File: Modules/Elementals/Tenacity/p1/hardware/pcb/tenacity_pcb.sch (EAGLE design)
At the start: 25 parts, among them J1 EURO_POWER, J2 WQP-PJ398SM6, J3 WQP-PJ398SM6, J4 WQP-PJ398SM6, J5 WQP-PJ398SM6, J6 WQP-PJ398SM6, J7 WQP-PJ398SM6, J8 WQP-PJ398SM6, J9 WQP-PJ398SM6, U1 TL072P, U2 TL072P

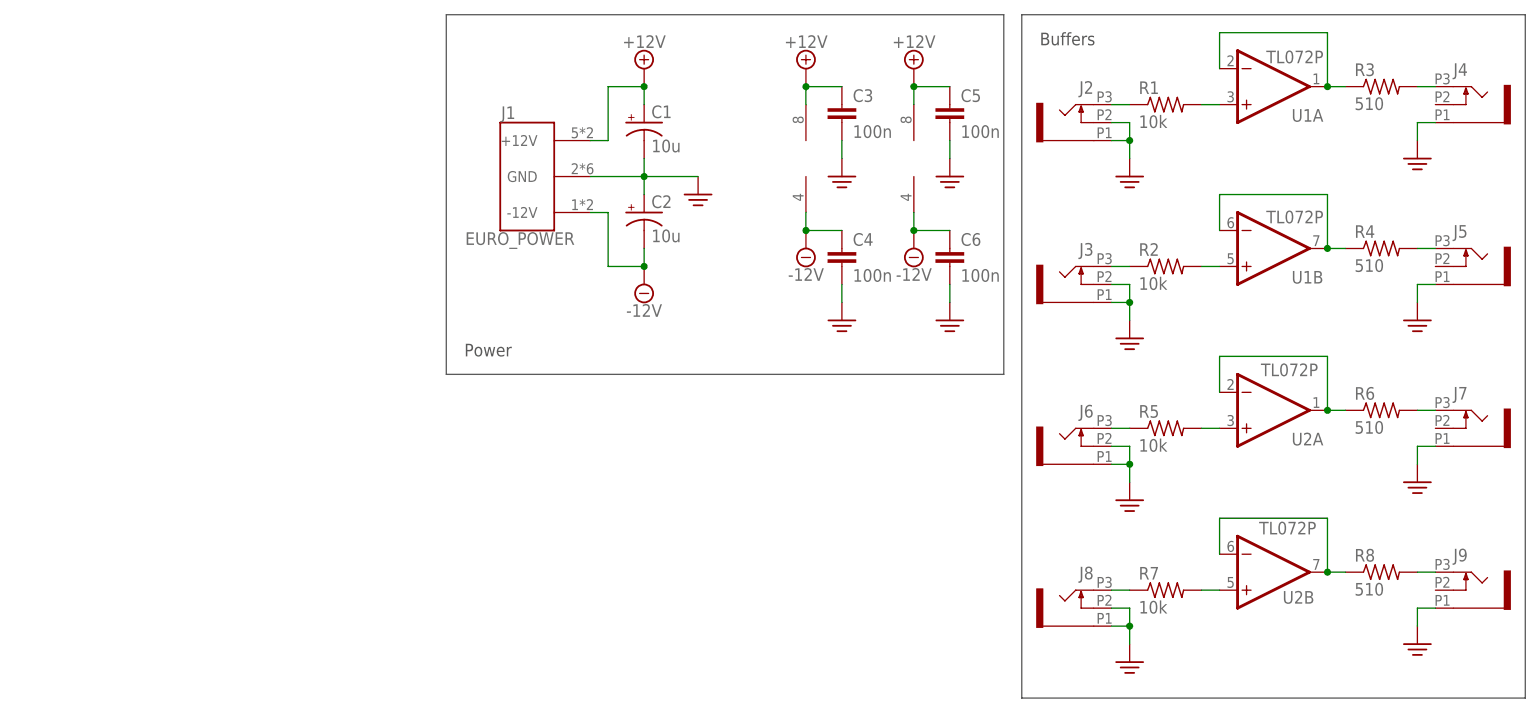
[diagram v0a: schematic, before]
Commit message: Finalized tenacity p1
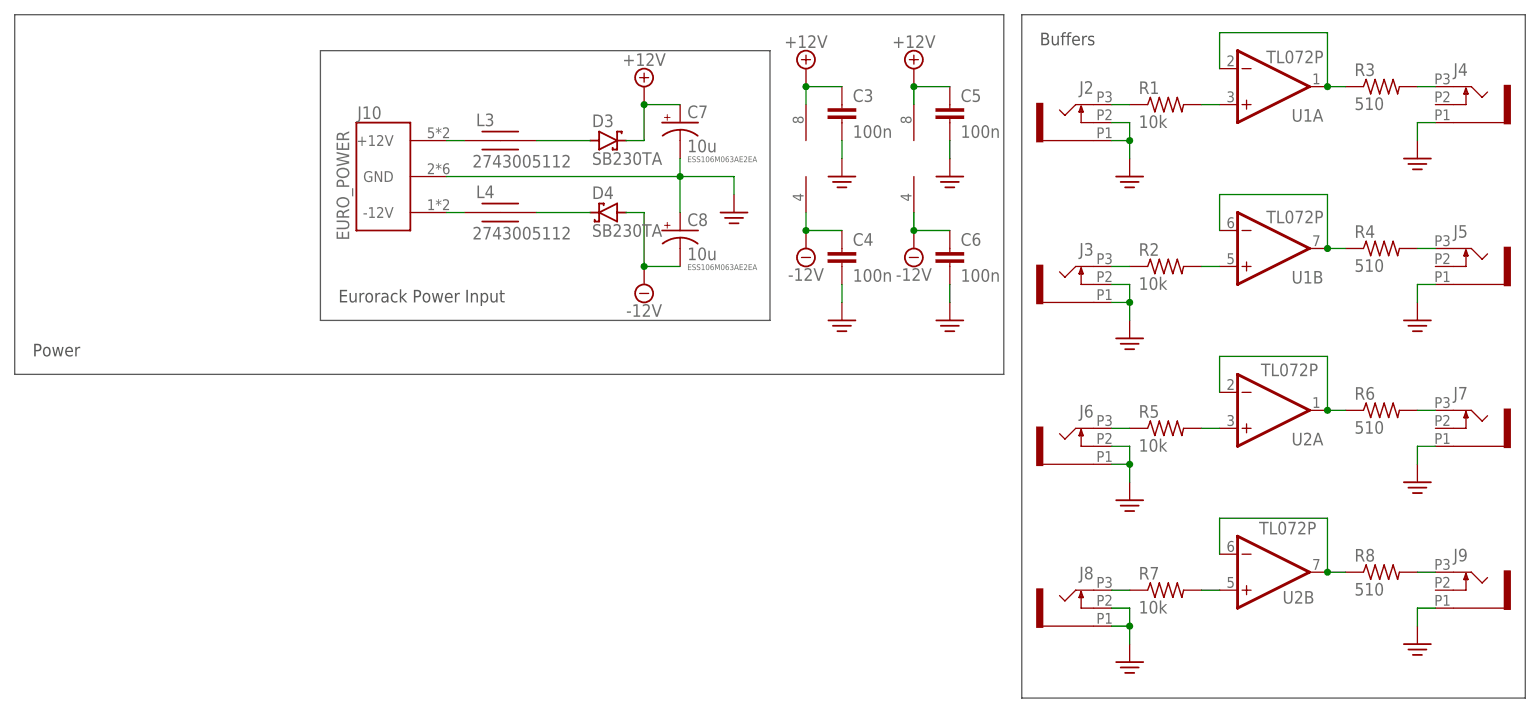
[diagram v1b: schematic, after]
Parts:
- removed C1, C2: 10u, SonicAthame:CAP_POLLYTIC_V
- removed J1: EURO_POWER, SonicAthame:EURO_POWER
- added C7, C8: 10u, SonicAthame:CAP_POLLYTIC_V
- added D3, D4: SB230TA, SonicAthame:SCHOTTKY_THT
- added J10: EURO_POWER, SonicAthame:EURO_POWER
- added L3, L4: 2743005112, SonicAthame:FERRITE_THT
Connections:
- new net N$21: D3.A, L3.P$2
- new net N$22: D4.C, L4.P$2
- new net N$23: J10.-12V, L4.P$1
- new net N$24: J10.+12V, L3.P$1
- net +12V: now also C7.+, D3.C; no longer C1.+, J1.+12V
- net -12V: now also C8.-, D4.A; no longer C2.-, J1.-12V
- net GND: now also C7.-, C8.+, J10.GND; no longer C1.-, C2.+, J1.GND
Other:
- note added: "ESS106M063AE2EA"
- note added: "Eurorack Power Input"
